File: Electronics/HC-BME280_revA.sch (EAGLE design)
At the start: 40 parts, among them SW1 SWITCH_SLIDE, T2 AO3401, U1 ATMEGA328-20P, U2 NRF24L01, U3 BME280, U4 OLED128X64, U5 BCO35

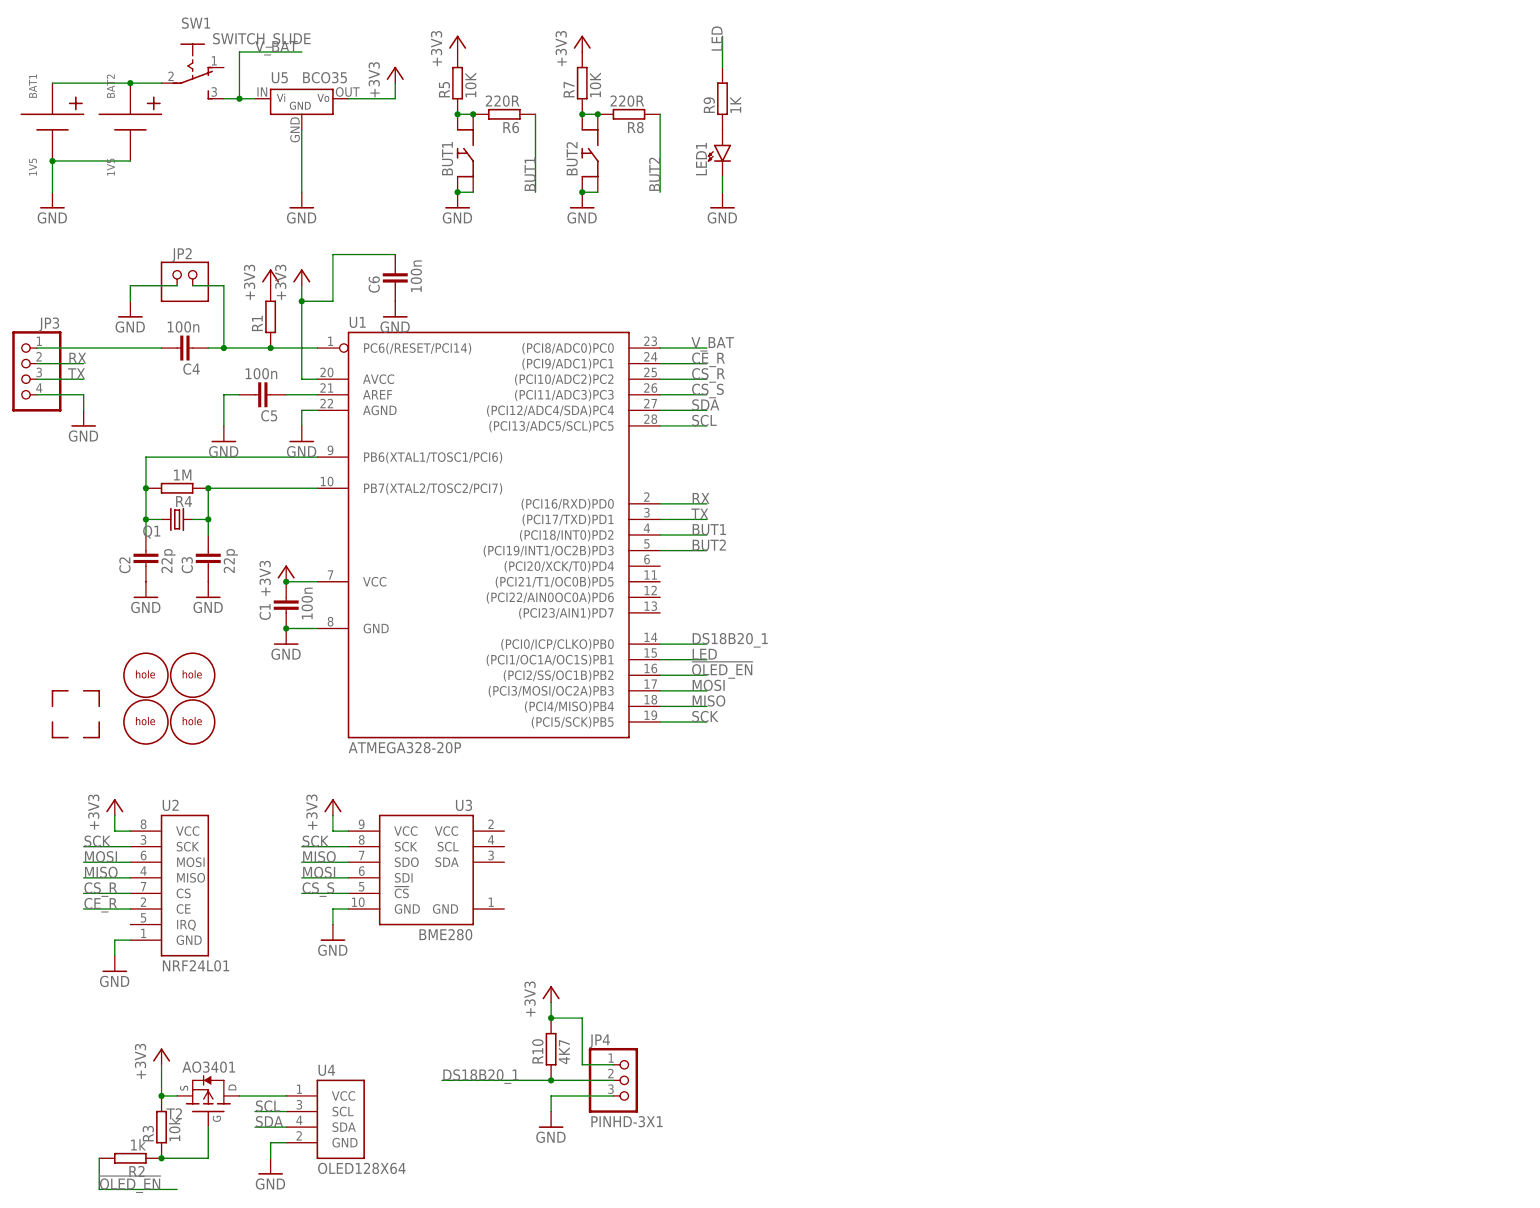
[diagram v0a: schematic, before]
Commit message: modified: minor changes in schematics and PCB
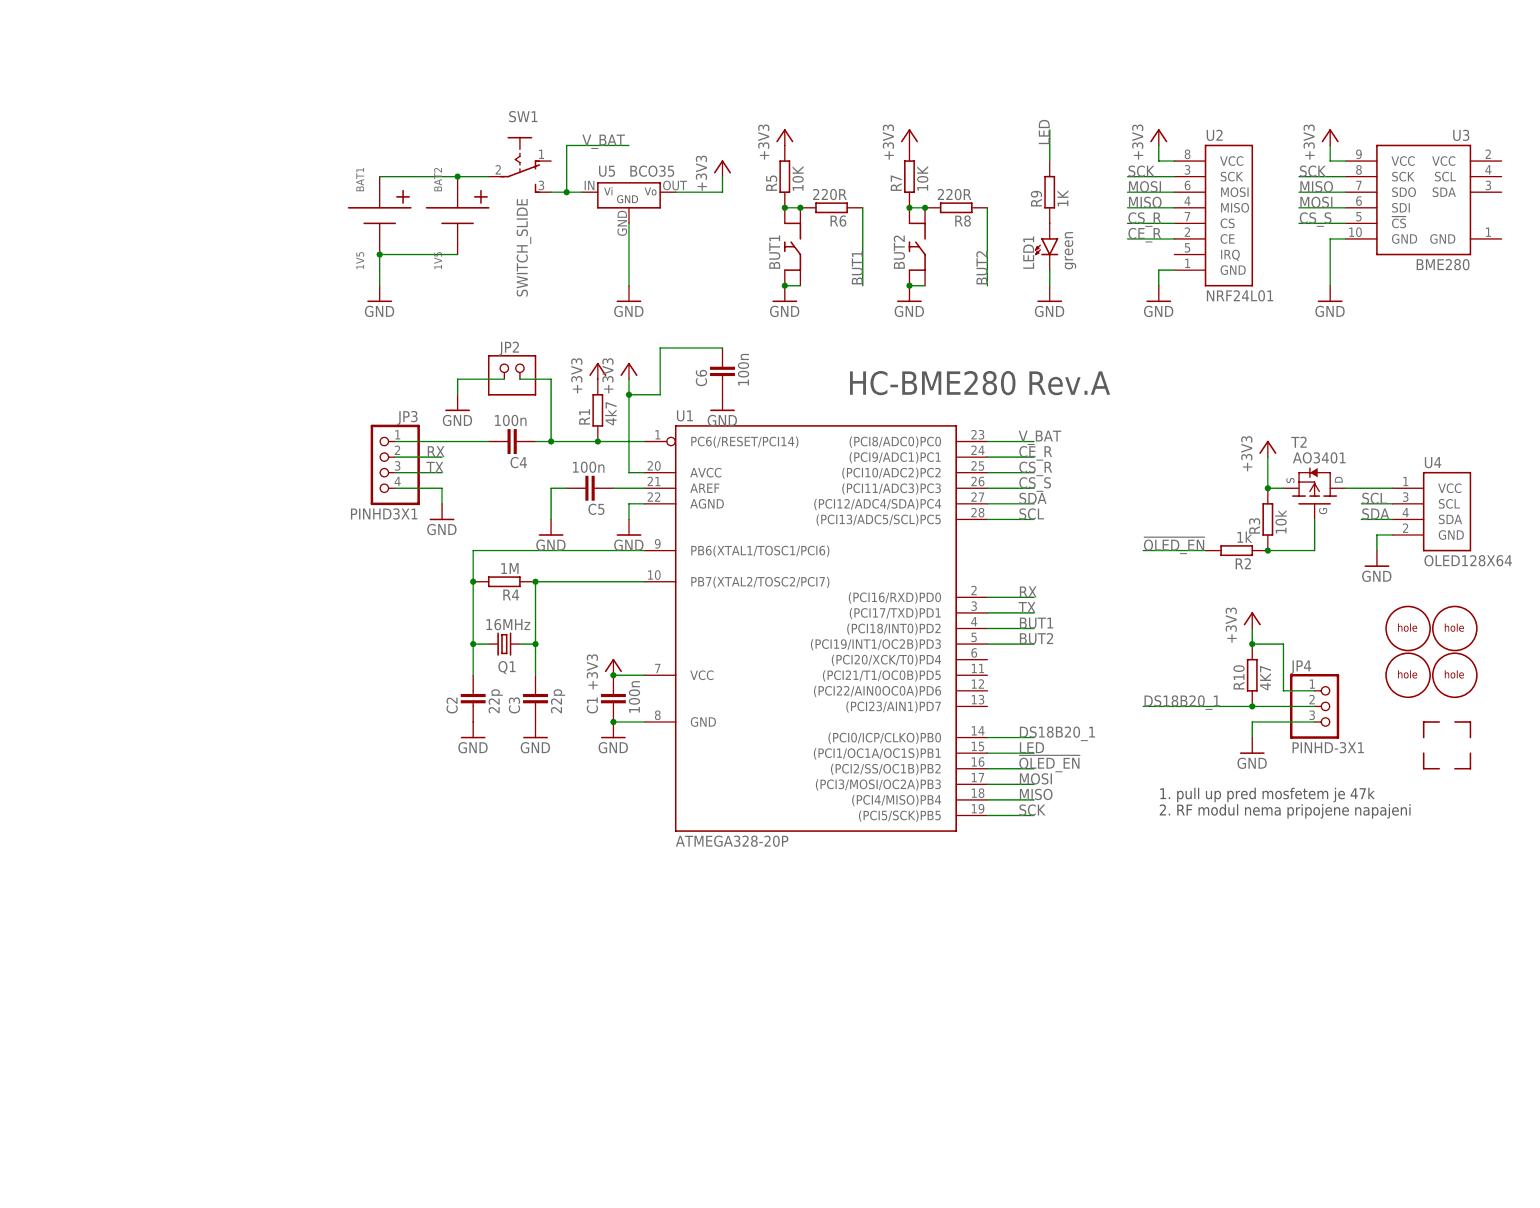
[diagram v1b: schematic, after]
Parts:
- JP2: value PINHD-2X1 -> PINHD2X1
- JP3: value (none) -> PINHD3X1
- LED1: value (none) -> green
- Q1: value (none) -> 16MHz
- R1: value (none) -> 4k7
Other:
- note added: "1. pull up pred mosfetem je 47k 2. RF modul nema pripojene napajeni"
- note added: "HC-BME280 Rev.A"
- moved on the sheet: BAT1, BAT2, BUT1, BUT2, C1, C2, C3, C4, C5, C6, JP2, JP3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
